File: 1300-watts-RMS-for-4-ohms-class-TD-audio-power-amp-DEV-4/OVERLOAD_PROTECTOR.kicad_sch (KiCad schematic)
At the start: 47 parts, among them Q901 2N5401, Q902 2N5551, Q903 TIP41C, U901 RC4558

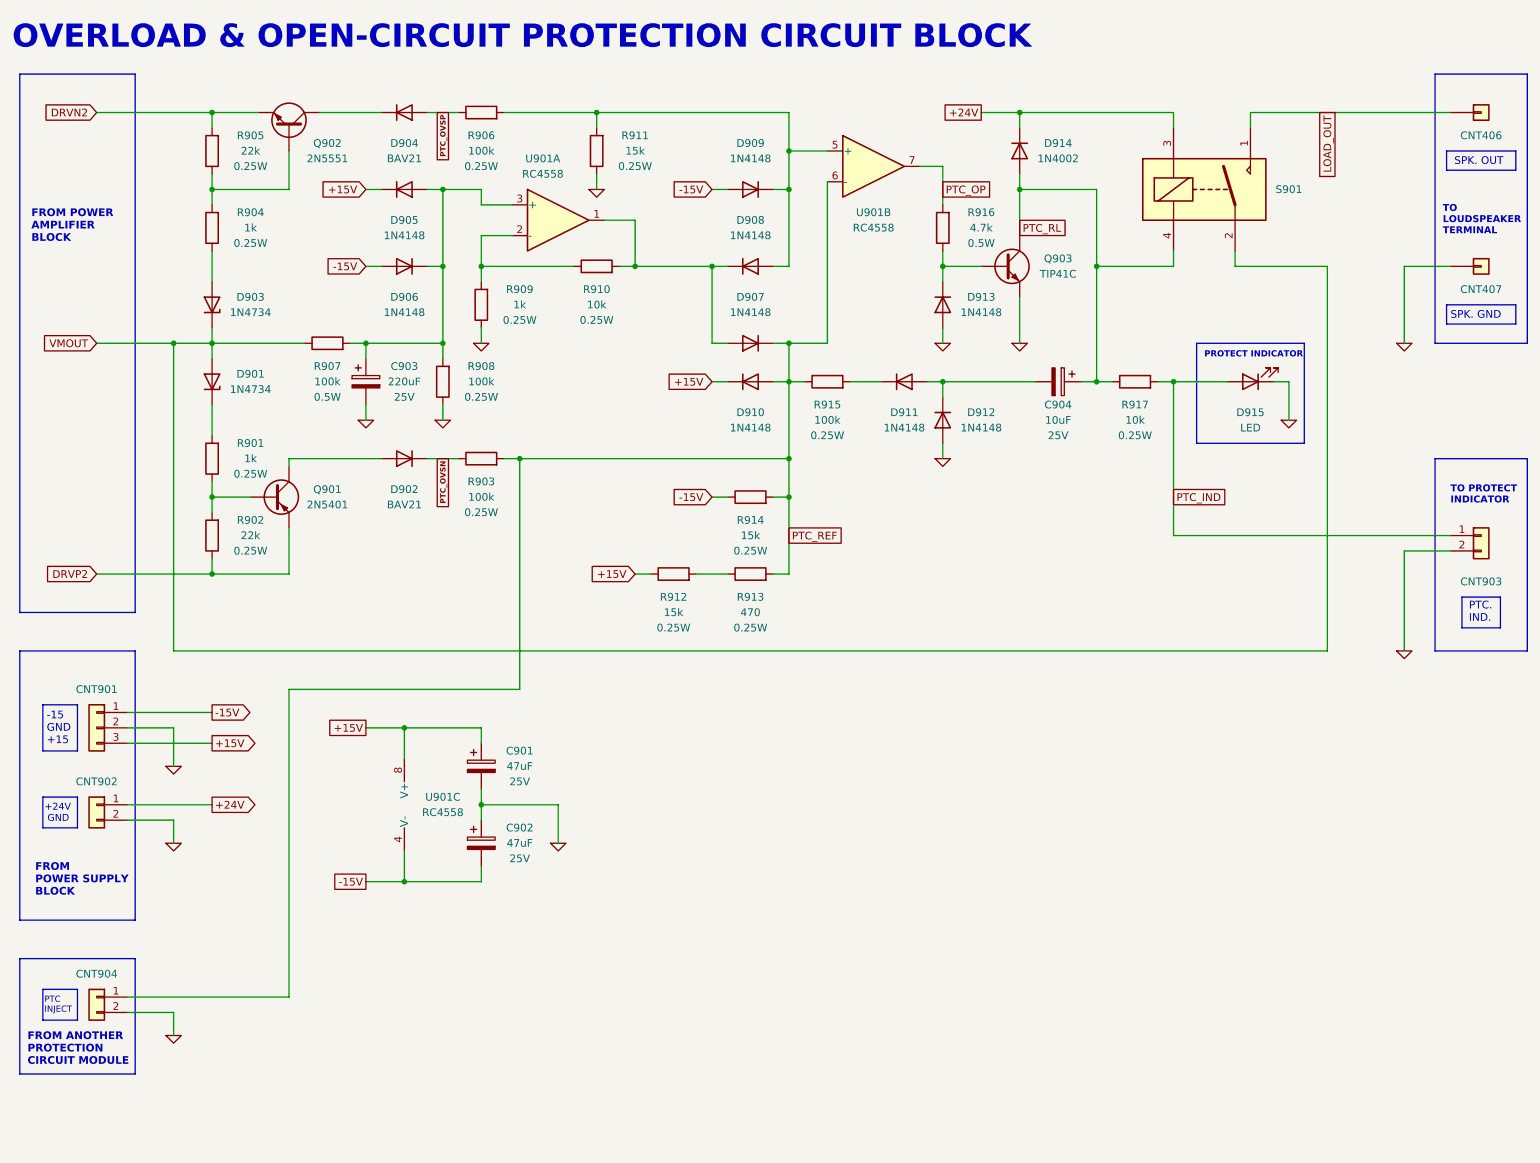
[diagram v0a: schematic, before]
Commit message: Update Tue Sep 13 06:42:19 AM WIB 2022
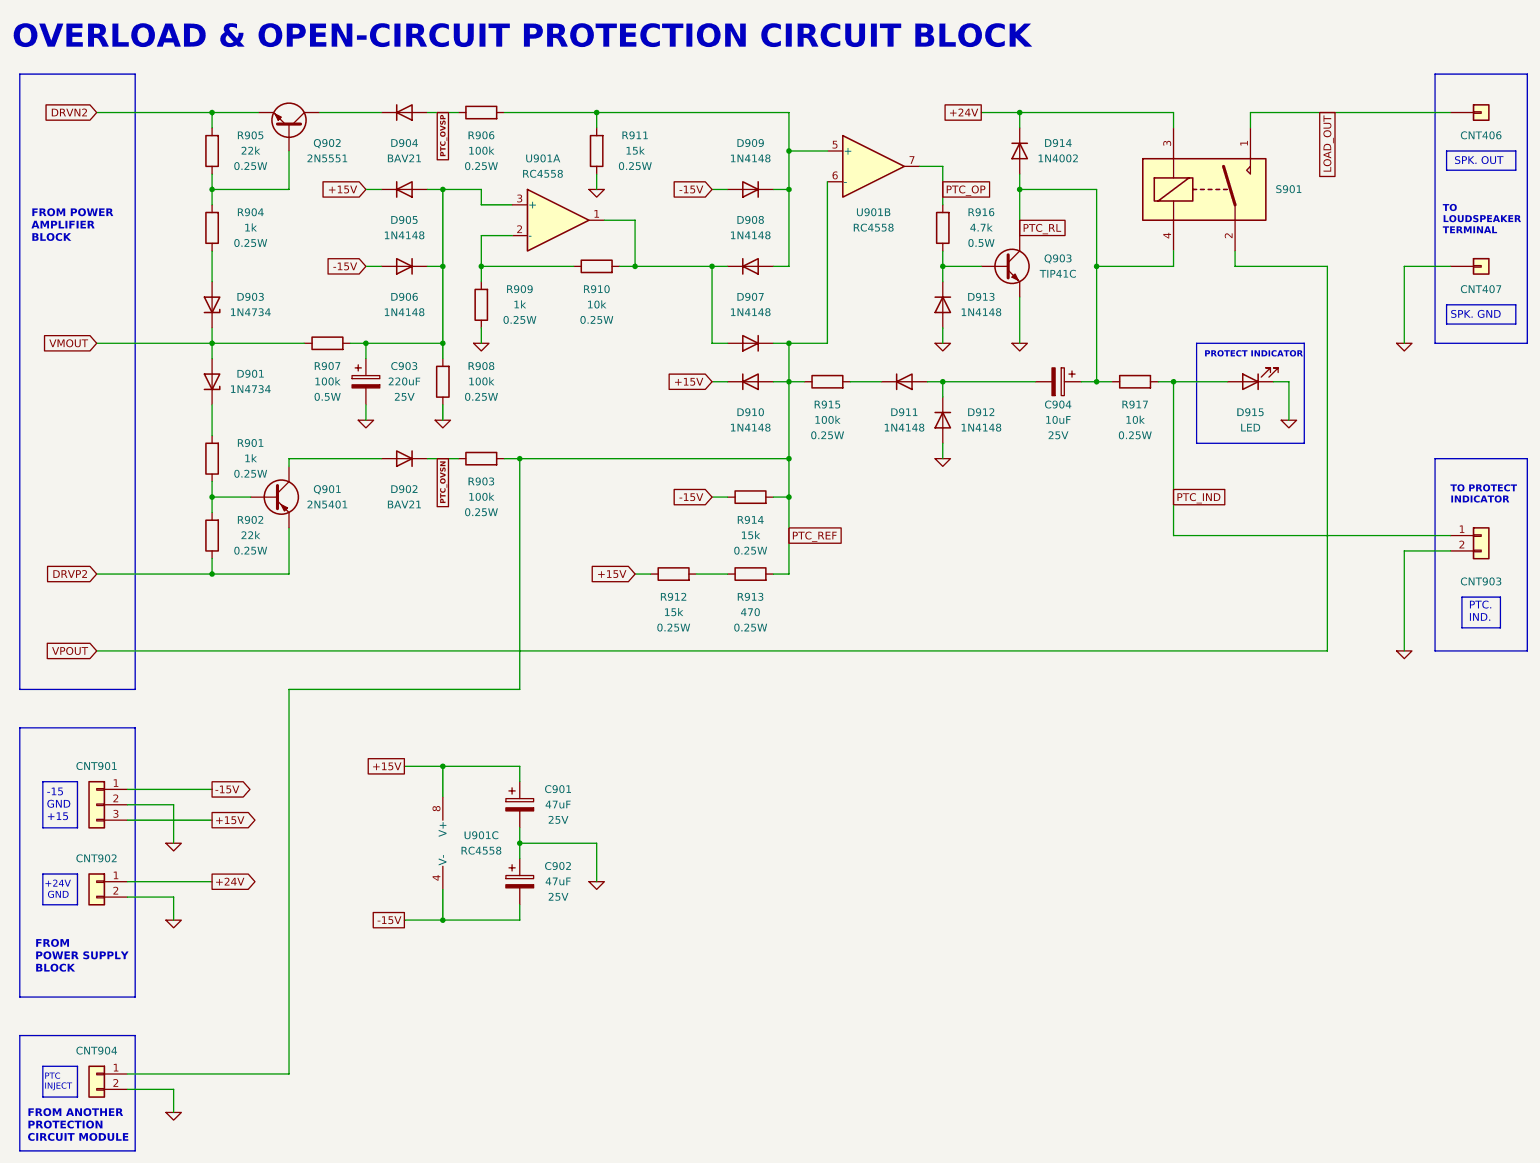
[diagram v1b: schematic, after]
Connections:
- net VMOUT: no longer S901.2
- new net VPOUT: S901.2
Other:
- moved on the sheet: C901, C902, CNT901, CNT902, CNT904, U901C
